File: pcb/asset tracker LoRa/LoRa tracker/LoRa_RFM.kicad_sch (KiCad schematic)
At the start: 9 parts, among them CON3 jtag, U8 murattaLora

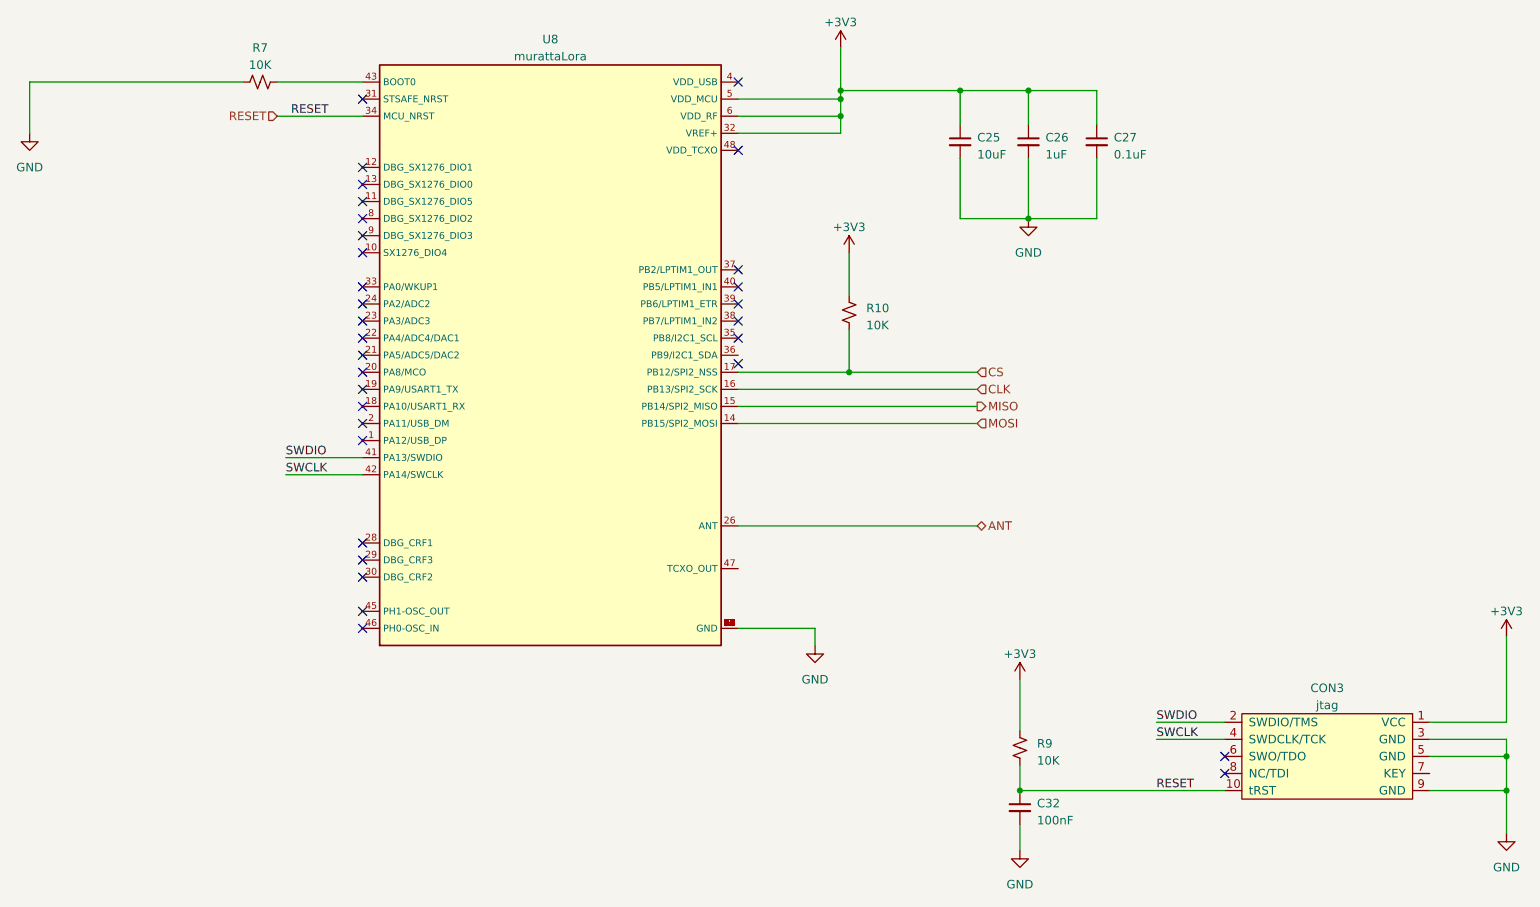
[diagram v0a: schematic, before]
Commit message: remake
remake 2 van de print
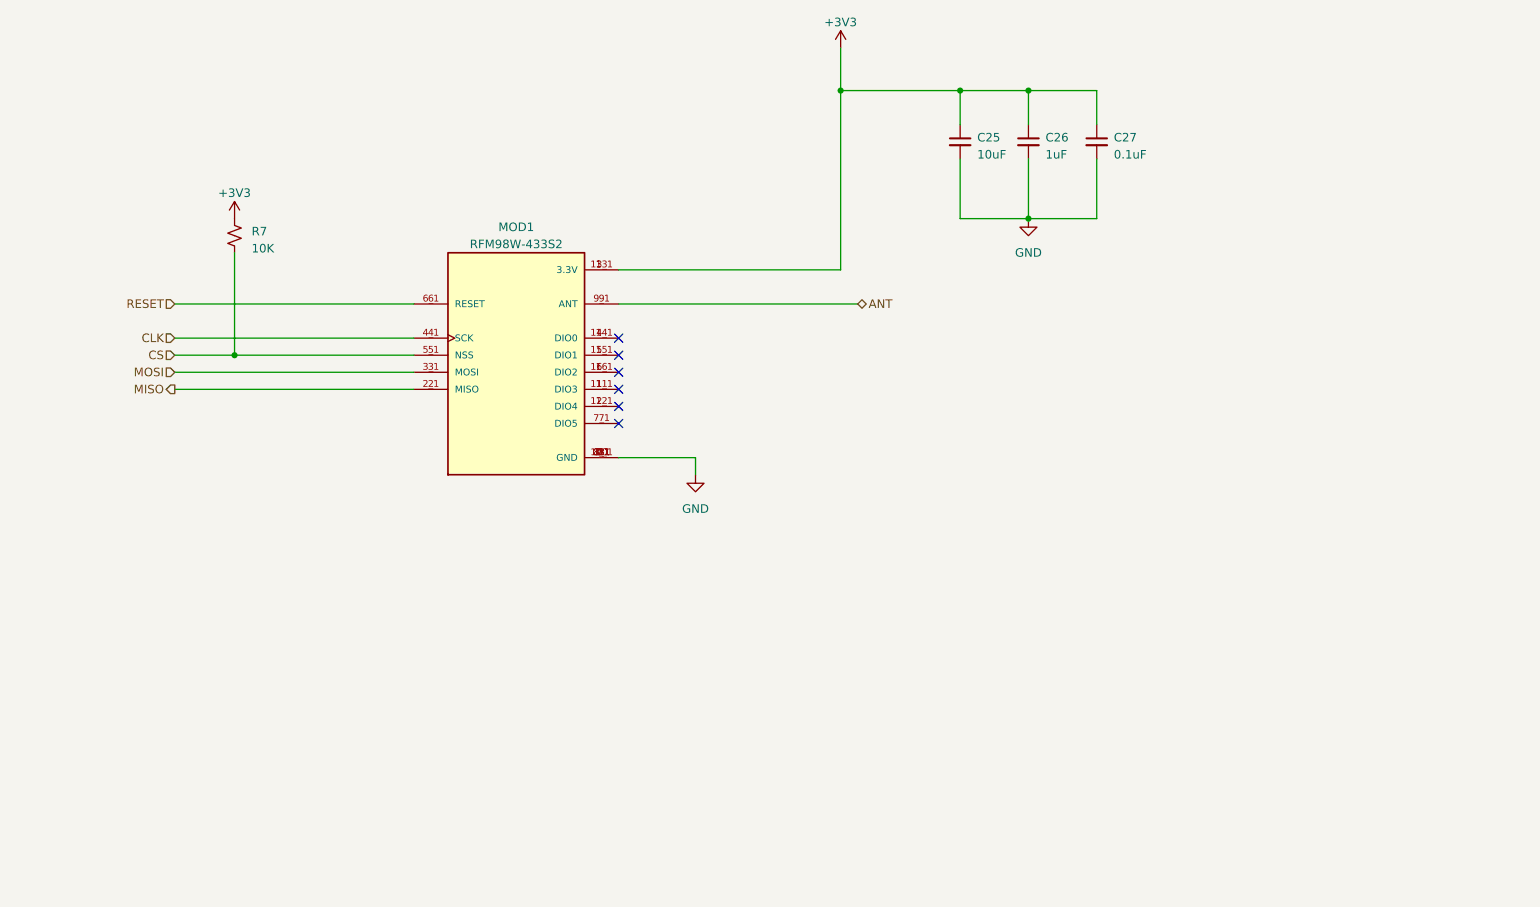
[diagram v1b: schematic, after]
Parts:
- removed C32: 100nF, vanalles:0603, symbol Device:C_Small
- removed CON3: jtag, connectors_user:Tag-Connect_TC2050-IDC-FP_2x05_P1.27mm_Vertical, symbol conectors:jtag
- removed R10, R9: 10K, vanalles:0603RL, symbol Device:R_Small_US
- removed U8: murattaLora, Module:XCVR_CMWX1ZZABZ-078, symbol modulles:murattaLora
- added MOD1: RFM98W-433S2, Module:XCVR_RFM98W-433S2, symbol RFM98W-433S2:RFM98W-433S2
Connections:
- net +3V3: now also R7.1, MOD1.13 (3.3V), MOD1.13_1 (3.3V)
- net ANT: now also MOD1.9 (ANT), MOD1.9_1 (ANT)
- net CLK: now also MOD1.4 (SCK), MOD1.4_1 (SCK)
- net CS: now also R7.2, MOD1.5 (NSS), MOD1.5_1 (NSS)
- net GND: now also MOD1.1 (GND), MOD1.10 (GND), MOD1.10_1 (GND), MOD1.1_1 (GND), MOD1.8 (GND), MOD1.8_1 (GND); no longer R7.1
- net MISO: now also MOD1.2 (MISO), MOD1.2_1 (MISO)
- net MOSI: now also MOD1.3 (MOSI), MOD1.3_1 (MOSI)
- net RESET: now also MOD1.6 (RESET), MOD1.6_1 (RESET)
- new net: MOD1.11 (DIO3), MOD1.11_1 (DIO3)
- new net: MOD1.12 (DIO4), MOD1.12_1 (DIO4)
- new net: MOD1.14 (DIO0), MOD1.14_1 (DIO0)
- new net: MOD1.15 (DIO1), MOD1.15_1 (DIO1)
- new net: MOD1.16 (DIO2), MOD1.16_1 (DIO2)
- new net: MOD1.7 (DIO5), MOD1.7_1 (DIO5)
- no-connect marks 32 -> 6
